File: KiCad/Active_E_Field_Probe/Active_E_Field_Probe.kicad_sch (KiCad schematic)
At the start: 10 parts

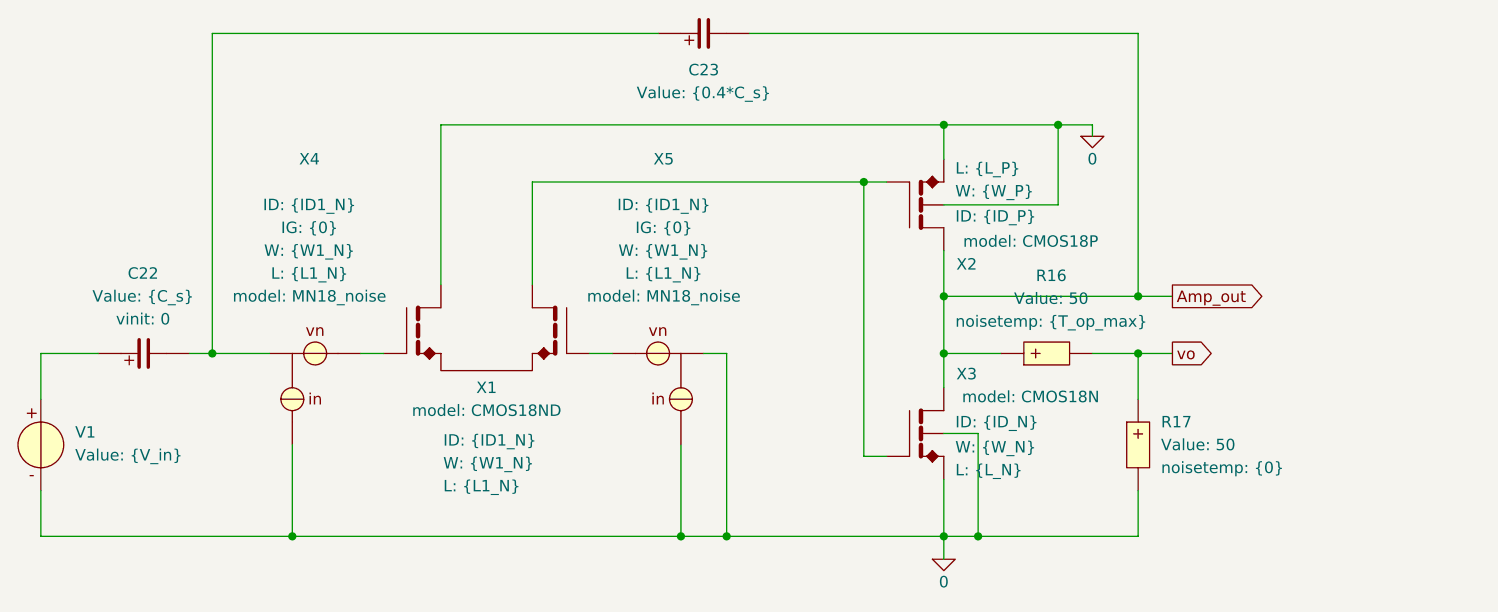
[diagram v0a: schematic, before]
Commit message: stuff
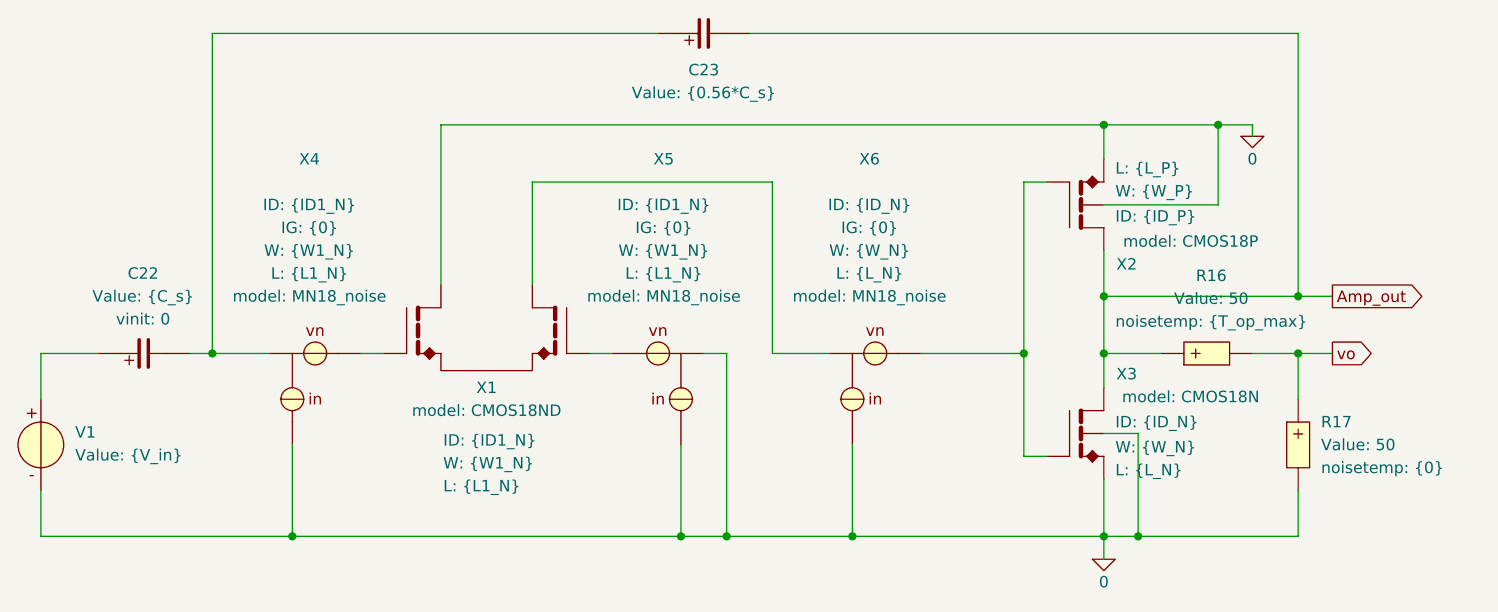
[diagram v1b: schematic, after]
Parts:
- added X6: ~, symbol SLiCAP:M_noise
- C23: value {0.4*C_s} -> {0.56*C_s}
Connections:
- net 0: now also X6.2 (comm)
- net at X2.2 (G), X3.2 (G): now also X6.3 (int); no longer X1.2 (D2)
- new net: X1.2 (D2), X6.1 (ext)
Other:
- moved on the sheet: R16, R17, X2, X3
